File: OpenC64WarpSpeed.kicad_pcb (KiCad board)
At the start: 2 copper layers, 58.4 x 61.7 mm, 17 parts, among them P1 C64-Exp-Port, SW1 SW_C64_C128, SW2 SW_Push, U1 74LS109, U2 27512

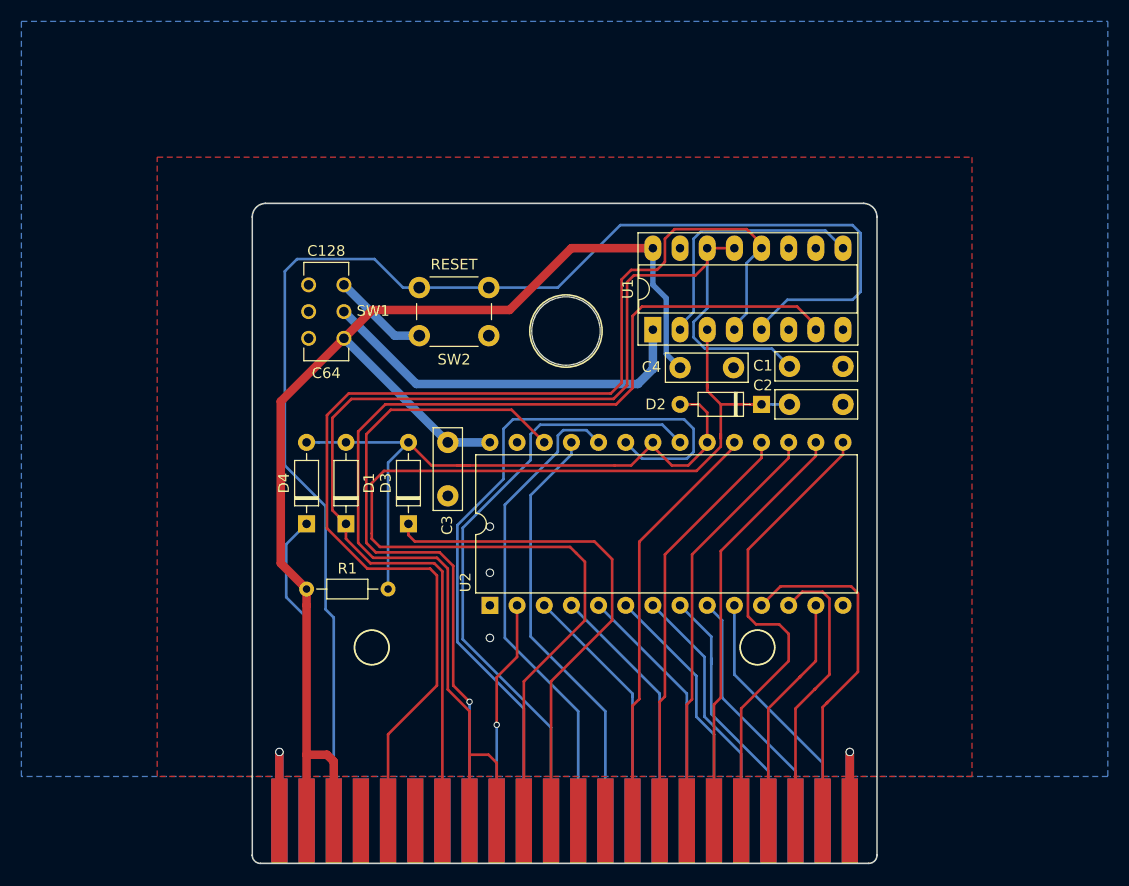
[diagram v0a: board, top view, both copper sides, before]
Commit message: Almost there
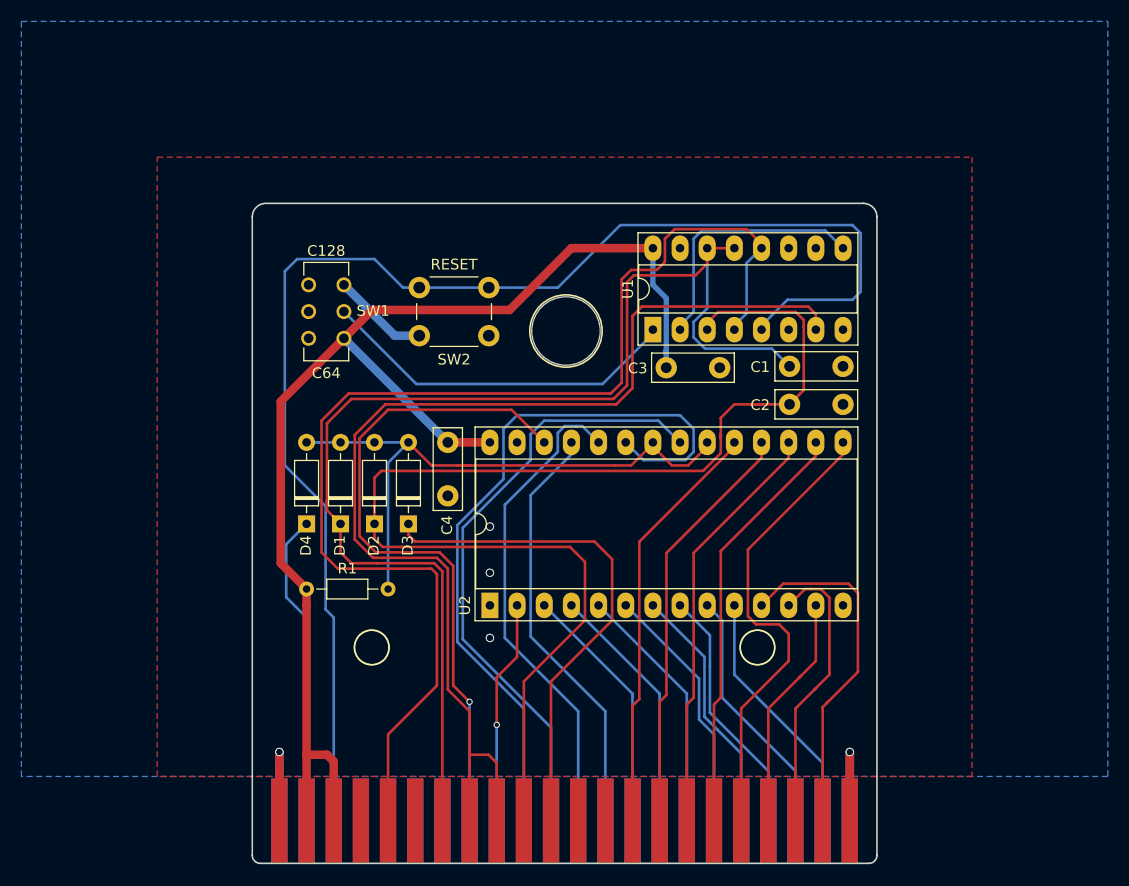
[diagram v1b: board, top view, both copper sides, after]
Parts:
- U2: footprint Package_DIP:DIP-28_W15.24mm -> Package_DIP:DIP-28_W15.24mm_Socket_LongPads
- moved D2 37.9 mm to (71.1, 97.8), turned to 90 degrees
- moved C3 1.29 mm to (98.4, 83.2)
- moved D1 0.51 mm to (67.9, 97.8)
- renumbered C4 to C3, C3 to C4
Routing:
- net Net-(C2-Pad1): track 106.3 -> 116.8 mm
- net Net-(D1-Pad2): track 62.9 -> 57.2 mm
- net Net-(P1-Pad5): track 112.0 -> 114.1 mm
- net Net-(SW1-Pad2): track 36.0 -> 34.0 mm
- net Net-(C1-Pad1): track 115.1 -> 116.9 mm
- net Net-(P1-Pad8): track 105.3 -> 106.2 mm
- net /a13: track 62.5 -> 63.2 mm
- net /a2: track 24.1 -> 23.6 mm
